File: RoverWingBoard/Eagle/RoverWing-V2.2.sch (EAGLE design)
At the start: 90 parts, among them J1 XT30UPB-M, J10 HEADER-3X04, J11 HEADER-3X06ANGLE, J12 HEADER-2X16, J13 HEADER-2X12, J14 DF13-4P-1.25DSA, J15 DF13-6P-1.25DSA, J16 HEADER-SH-4P, J2 HEADER-VH, J3 HEADER-VH, J4 HEADER-PH-4P, J5 HEADER-PH-4P, J6 HEADER-PH-4P, J7 HEADER-PH-4P, J8 HEADER-PH-4P, J9 HEADER-PH-3P, SW1 SW-TACTILE-4.5X4.5_SMD, U1 ATSAMD21G, U2 TPS54531, U3 PMIC-AZ1117EH-3.3, U4 ICM-42605, U5 DRV8871, U6 DRV8871, U7 74AHCT1G125DBV

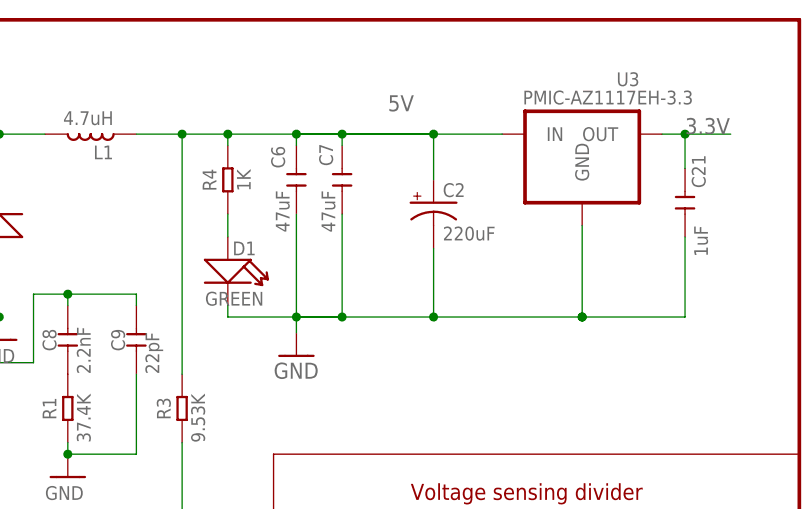
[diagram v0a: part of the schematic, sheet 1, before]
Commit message: board version 2.2
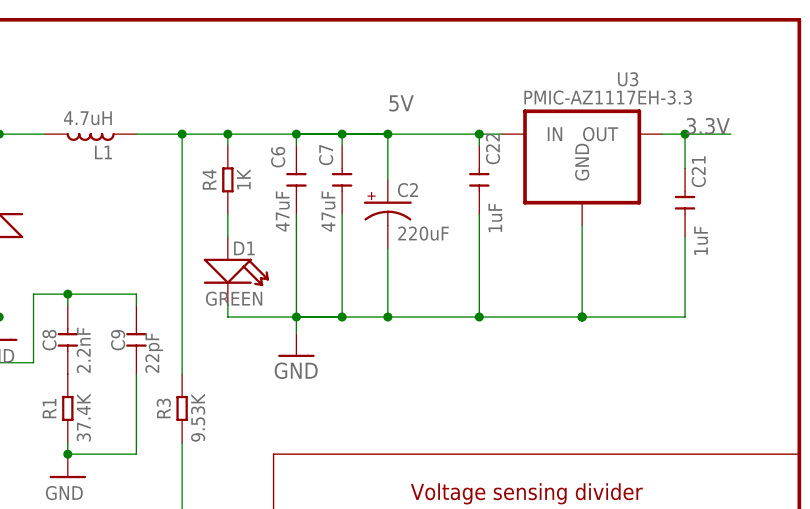
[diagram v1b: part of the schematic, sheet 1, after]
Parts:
- added C22: 1uF, RoverWing-V1.5:CAP-CERAMIC-SMD0603
- C21: device RoverWing-V1.5:CAP-CERAMIC-SMD0805 -> RoverWing-V1.5:CAP-CERAMIC-SMD0603
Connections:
- net 5V: now also C22.2
- net GND: now also C22.1
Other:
- moved on the sheet: C2
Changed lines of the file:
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@@
 <part name="C19" library="RoverWing-V1.5" deviceset="CAP-CERAMIC-SMD" device="0603" value="100nF"/>
 <part name="C20" library="RoverWing-V1.5" deviceset="CAP-CERAMIC-SMD" device="0603" value="100nF"/>
-<part name="C21" library="RoverWing-V1.5" deviceset="CAP-CERAMIC-SMD" device="0805" value="1uF"/>
+<part name="C21" library="RoverWing-V1.5" deviceset="CAP-CERAMIC-SMD" device="0603" value="1uF"/>
 <part name="C14" library="RoverWing-V1.5" deviceset="CAP-CERAMIC-SMD" device="0603" value="100nF"/>
 <part name="C13" library="RoverWing-V1.5" deviceset="CAP-CERAMIC-SMD" device="0603" value="100nF"/>
@@
 <part name="D3" library="RoverWing-V1.5" deviceset="SMD-DIODE-SCHOTTKY" device="DO-214AC" package3d_urn="urn:adsk.eagle:package:43452/2"/>
 <part name="GND3" library="RoverWing-V1.5" deviceset="GND" device=""/>
+<part name="C22" library="RoverWing-V1.5" deviceset="CAP-CERAMIC-SMD" device="0603" value="1uF"/>
 </parts>
 <sheets>
@@
 <attribute name="NAME" x="115.57" y="8.89" size="1.524" layer="95" font="vector" ratio="10"/>
 </instance>
-<instance part="C2" gate="G$1" x="208.28" y="165.1" smashed="yes">
-<attribute name="NAME" x="209.296" y="165.735" size="1.524" layer="95" ratio="10"/>
-<attribute name="VALUE" x="209.296" y="160.909" size="1.524" layer="96" ratio="10"/>
+<instance part="C2" gate="G$1" x="203.2" y="165.1" smashed="yes">
+<attribute name="NAME" x="204.216" y="165.735" size="1.524" layer="95" ratio="10"/>
+<attribute name="VALUE" x="204.216" y="160.909" size="1.524" layer="96" ratio="10"/>
 </instance>
 <instance part="U4" gate="G$1" x="203.2" y="78.74" smashed="yes">
@@
 <instance part="GND3" gate="1" x="160.02" y="149.86" smashed="yes">
 <attribute name="VALUE" x="157.48" y="147.32" size="1.524" layer="96" ratio="10"/>
+</instance>
+<instance part="C22" gate="G$1" x="213.36" y="167.64" smashed="yes" rot="R90">
+<attribute name="NAME" x="214.122" y="172.974" size="1.524" layer="95" ratio="10" rot="R270"/>
+<attribute name="VALUE" x="214.376" y="165.1" size="1.524" layer="96" ratio="10" rot="R270"/>
 </instance>
 </instances>
@@
 <pinref part="C21" gate="G$1" pin="1"/>
 <pinref part="U3" gate="G$1" pin="GND"/>
-<wire x1="193.04" y1="152.4" x2="208.28" y2="152.4" width="0.1524" layer="91"/>
-<wire x1="208.28" y1="152.4" x2="224.79" y2="152.4" width="0.1524" layer="91"/>
+<wire x1="193.04" y1="152.4" x2="203.2" y2="152.4" width="0.1524" layer="91"/>
+<wire x1="203.2" y1="152.4" x2="213.36" y2="152.4" width="0.1524" layer="91"/>
+<wire x1="213.36" y1="152.4" x2="224.79" y2="152.4" width="0.1524" layer="91"/>
 <wire x1="224.79" y1="162.56" x2="224.79" y2="152.4" width="0.1524" layer="91"/>
 <junction x="224.79" y="152.4"/>
@@
 <junction x="193.04" y="152.4"/>
 <wire x1="193.04" y1="152.4" x2="193.04" y2="150.622" width="0.1524" layer="91"/>
-<wire x1="208.28" y1="160.02" x2="208.28" y2="152.4" width="0.1524" layer="91"/>
-<junction x="208.28" y="152.4"/>
+<wire x1="203.2" y1="160.02" x2="203.2" y2="152.4" width="0.1524" layer="91"/>
+<junction x="203.2" y="152.4"/>
 <wire x1="193.04" y1="152.4" x2="185.42" y2="152.4" width="0.1524" layer="91"/>
 <wire x1="185.42" y1="152.4" x2="185.42" y2="153.67" width="0.1524" layer="91"/>
+<pinref part="C22" gate="G$1" pin="1"/>
+<wire x1="213.36" y1="163.83" x2="213.36" y2="152.4" width="0.1524" layer="91"/>
+<junction x="213.36" y="152.4"/>
 </segment>
 <segment>
@@
 <junction x="185.42" y="172.72"/>
 <pinref part="C2" gate="G$1" pin="+"/>
-<wire x1="208.28" y1="167.64" x2="208.28" y2="172.72" width="0.1524" layer="91"/>
+<wire x1="203.2" y1="167.64" x2="203.2" y2="172.72" width="0.1524" layer="91"/>
 <pinref part="U3" gate="G$1" pin="IN"/>
 <pinref part="C7" gate="G$1" pin="2"/>
 <wire x1="198.12" y1="171.45" x2="198.12" y2="172.72" width="0.1524" layer="91"/>
-<wire x1="198.12" y1="172.72" x2="215.9" y2="172.72" width="0.1524" layer="91"/>
+<wire x1="198.12" y1="172.72" x2="213.36" y2="172.72" width="0.1524" layer="91"/>
+<wire x1="213.36" y1="172.72" x2="215.9" y2="172.72" width="0.1524" layer="91"/>
 <wire x1="198.12" y1="172.72" x2="193.04" y2="172.72" width="0.1524" layer="91"/>
 <pinref part="C6" gate="G$1" pin="2"/>
 <wire x1="193.04" y1="171.45" x2="193.04" y2="172.72" width="0.1524" layer="91"/>
 <junction x="193.04" y="172.72"/>
-<wire x1="185.42" y1="172.72" x2="208.28" y2="172.72" width="0.1524" layer="91"/>
+<wire x1="185.42" y1="172.72" x2="203.2" y2="172.72" width="0.1524" layer="91"/>
 <label x="203.2" y="175.26" size="1.778" layer="95"/>
-<junction x="208.28" y="172.72"/>
-<wire x1="208.28" y1="172.72" x2="193.04" y2="172.72" width="0.1524" layer="91"/>
+<junction x="203.2" y="172.72"/>
+<wire x1="203.2" y1="172.72" x2="193.04" y2="172.72" width="0.1524" layer="91"/>
 <junction x="198.12" y="172.72"/>
-</segment>
-</net>
+<pinref part="C22" gate="G$1" pin="2"/>
+<wire x1="213.36" y1="171.45" x2="213.36" y2="172.72" width="0.1524" layer="91"/>
+<junction x="213.36" y="172.72"/>
+</segment>
+</net>
